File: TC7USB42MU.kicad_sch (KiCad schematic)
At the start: 5 parts, among them U2 TC7USB42MU

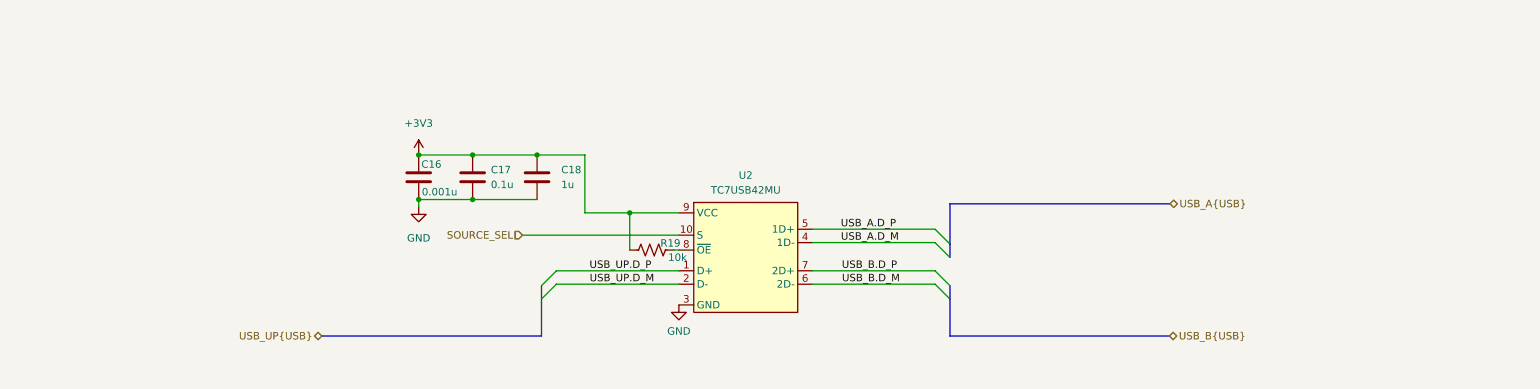
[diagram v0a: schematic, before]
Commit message: Pushing what i have now
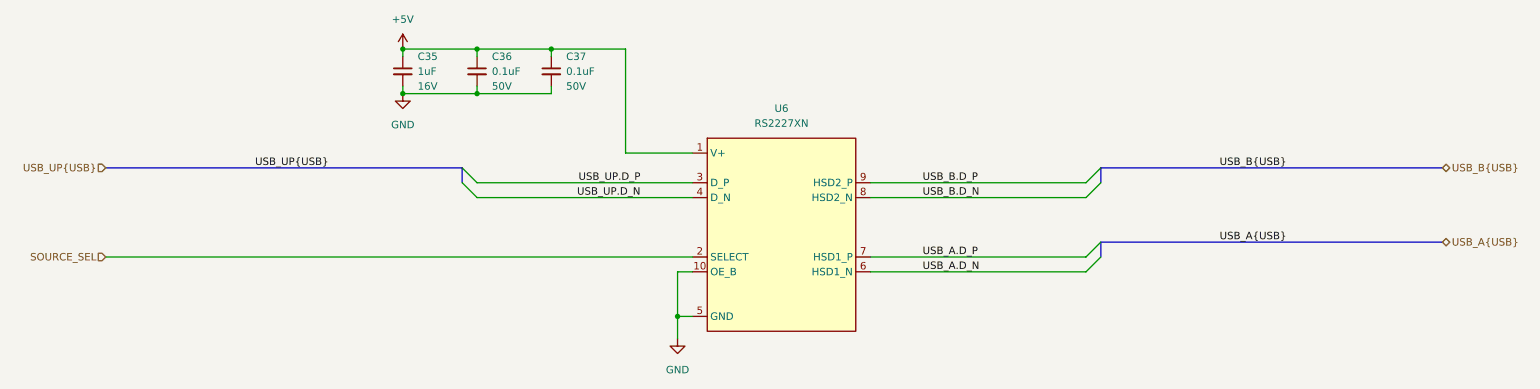
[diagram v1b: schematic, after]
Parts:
- removed C16: 0.001u, symbol Device:C
- removed C17: 0.1u, symbol Device:C
- removed C18: 1u, symbol Device:C
- removed R19: 10k, symbol Device:R_US
- removed U2: TC7USB42MU, symbol Misic:TC7USB42MU
- added C35: ${Capacitance}, Capacitor_SMD:C_0603_1608Metric_Pad1.08x0.95mm_HandSolder, symbol Rockerrobotics:Capacitors/1276-1034-1-ND
- added C36, C37: ${Capacitance}, Capacitor_SMD:C_0603_1608Metric_Pad1.08x0.95mm_HandSolder, symbol Rockerrobotics:Capacitors/1276-1935-1-ND
- added U6: ${MPN}, Package_SO:MSOP-10_3x3mm_P0.5mm, symbol Rockerrobotics:Integrated Circuits/3565-RS2227XNCT-ND
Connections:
- net GND: now also C35.2, C36.2, C37.2, U6.10 (OE_B), U6.5 (GND)
- net SOURCE_SEL: now also U6.2 (SELECT)
- net USB_A.D_P: now also U6.7 (HSD1_P)
- net USB_B.D_P: now also U6.9 (HSD2_P)
- net USB_UP.D_P: now also U6.3 (D_P)
- new net +5V: C35.1, C36.1, C37.1, U6.1 (V+)
- new net USB_A.D_N: U6.6 (HSD1_N)
- new net USB_B.D_N: U6.8 (HSD2_N)
- new net USB_UP.D_N: U6.4 (D_N)
